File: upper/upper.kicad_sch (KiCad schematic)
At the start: 22 parts, among them SW1 SW_Push, U1 RaspberryPi_Pico_W

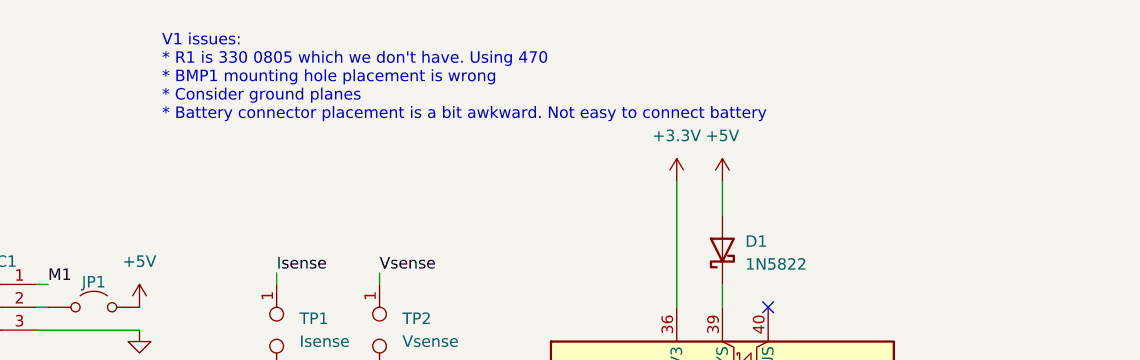
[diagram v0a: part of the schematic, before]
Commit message: Upper: Add to v1 issues list
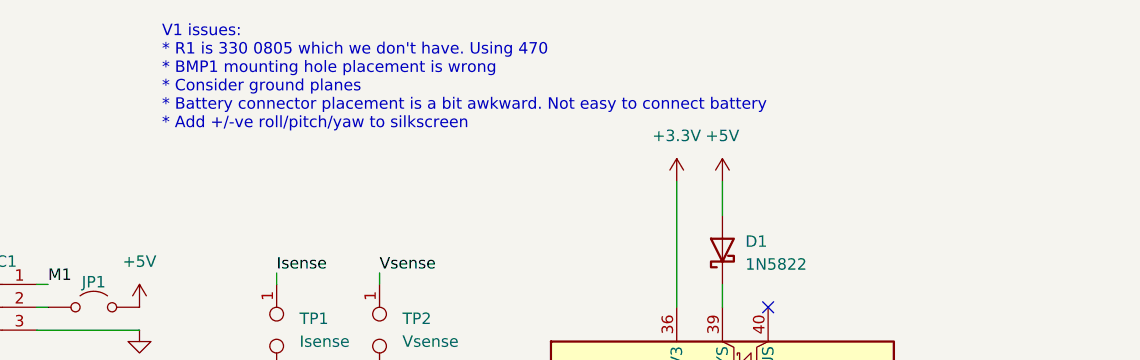
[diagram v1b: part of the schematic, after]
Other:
- note added: "V1 issues: * R1 is 330 0805 which we don't have. Using 470 * BMP1 mounting hole placement is wrong * Consider ground planes * Battery connector placement is a bit awkward. Not easy to connect battery * Add +/-ve roll/pitch/yaw to silkscreen"
- note removed: "V1 issues: * R1 is 330 0805 which we don't have. Using 470 * BMP1 mounting hole placement is wrong * Consider ground planes * Battery connector placement is a bit awkward. Not easy to connect battery"
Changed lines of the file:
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@@
 		)
 	)
-	(text "V1 issues:\n* R1 is 330 0805 which we don't have. Using 470\n* BMP1 mounting hole placement is wrong\n* Consider ground planes\n* Battery connector placement is a bit awkward. Not easy to connect battery"
+	(text "V1 issues:\n* R1 is 330 0805 which we don't have. Using 470\n* BMP1 mounting hole placement is wrong\n* Consider ground planes\n* Battery connector placement is a bit awkward. Not easy to connect battery\n* Add +/-ve roll/pitch/yaw to silkscreen"
 		(exclude_from_sim no)
 		(at 83.7795 26.6053 0)
